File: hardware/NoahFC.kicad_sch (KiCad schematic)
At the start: 44 parts, among them J1 ALE, J11 SCK, J12 MISO, J17 VTX, J18 RESET, J2 ELE, J3 CAM, J4 FTDI, J5 VCC, J6 THR, J7 PPM, J8 GPS, U1 ATmega328, U2 MPU-6050, U4 AMS1117-3.3, U5 MAX7456EUI+, U6 HMC5883L, Y1 16Mhz, Y2 27Mhz

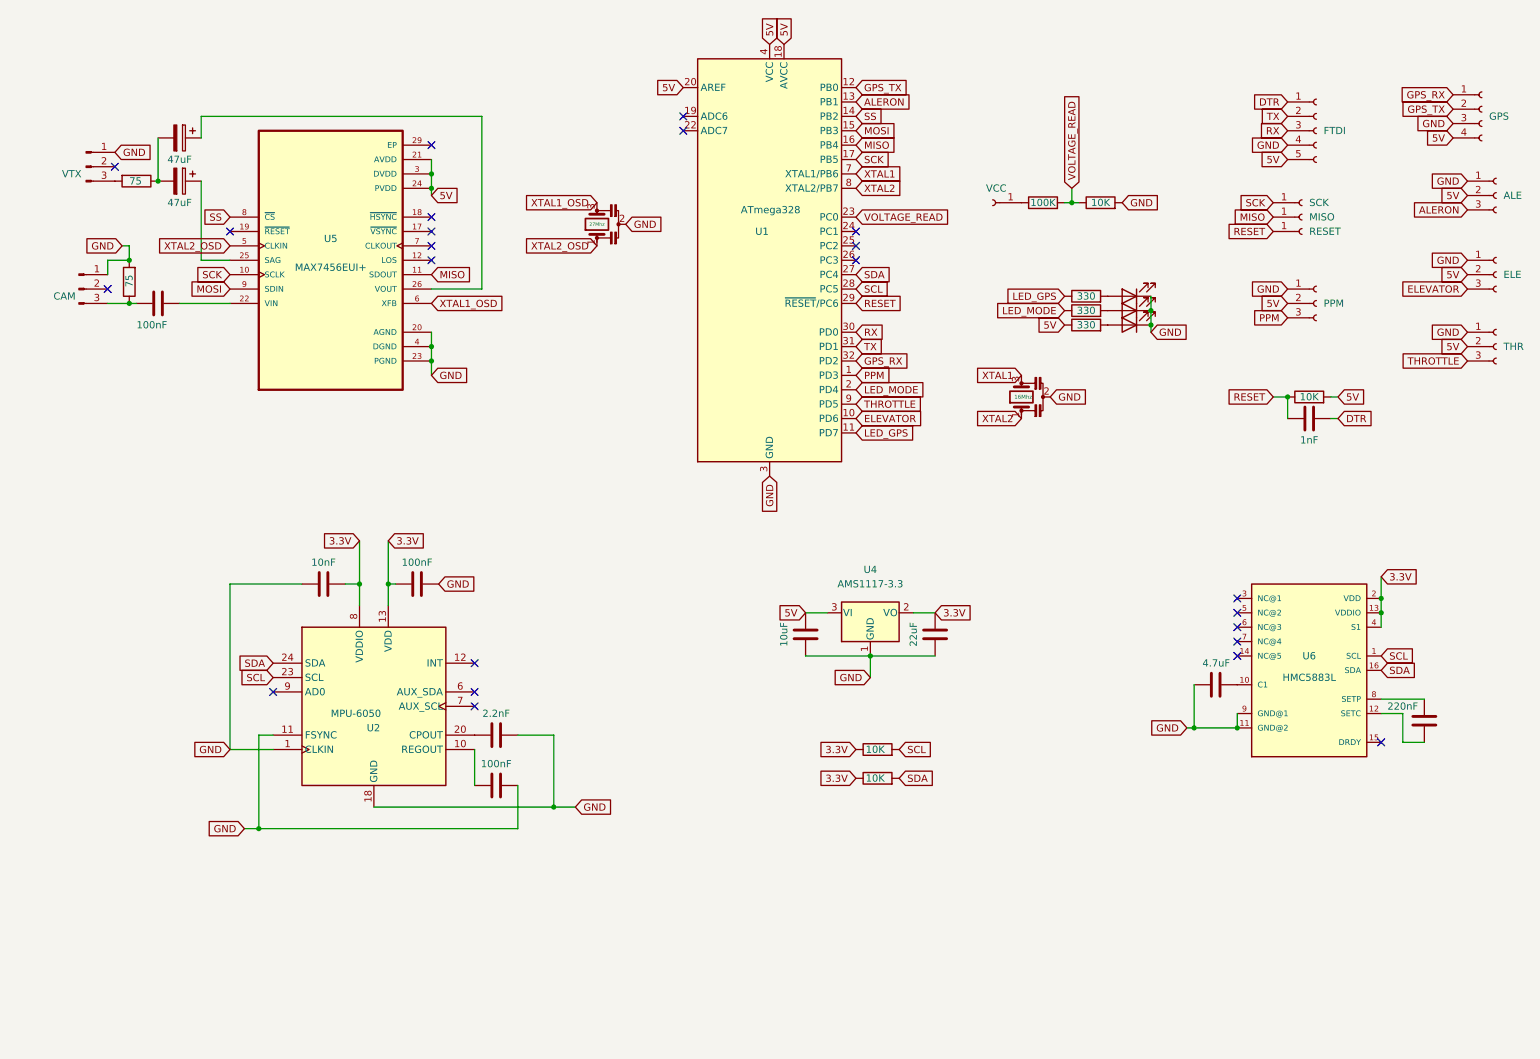
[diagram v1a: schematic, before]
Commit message: rev4 project
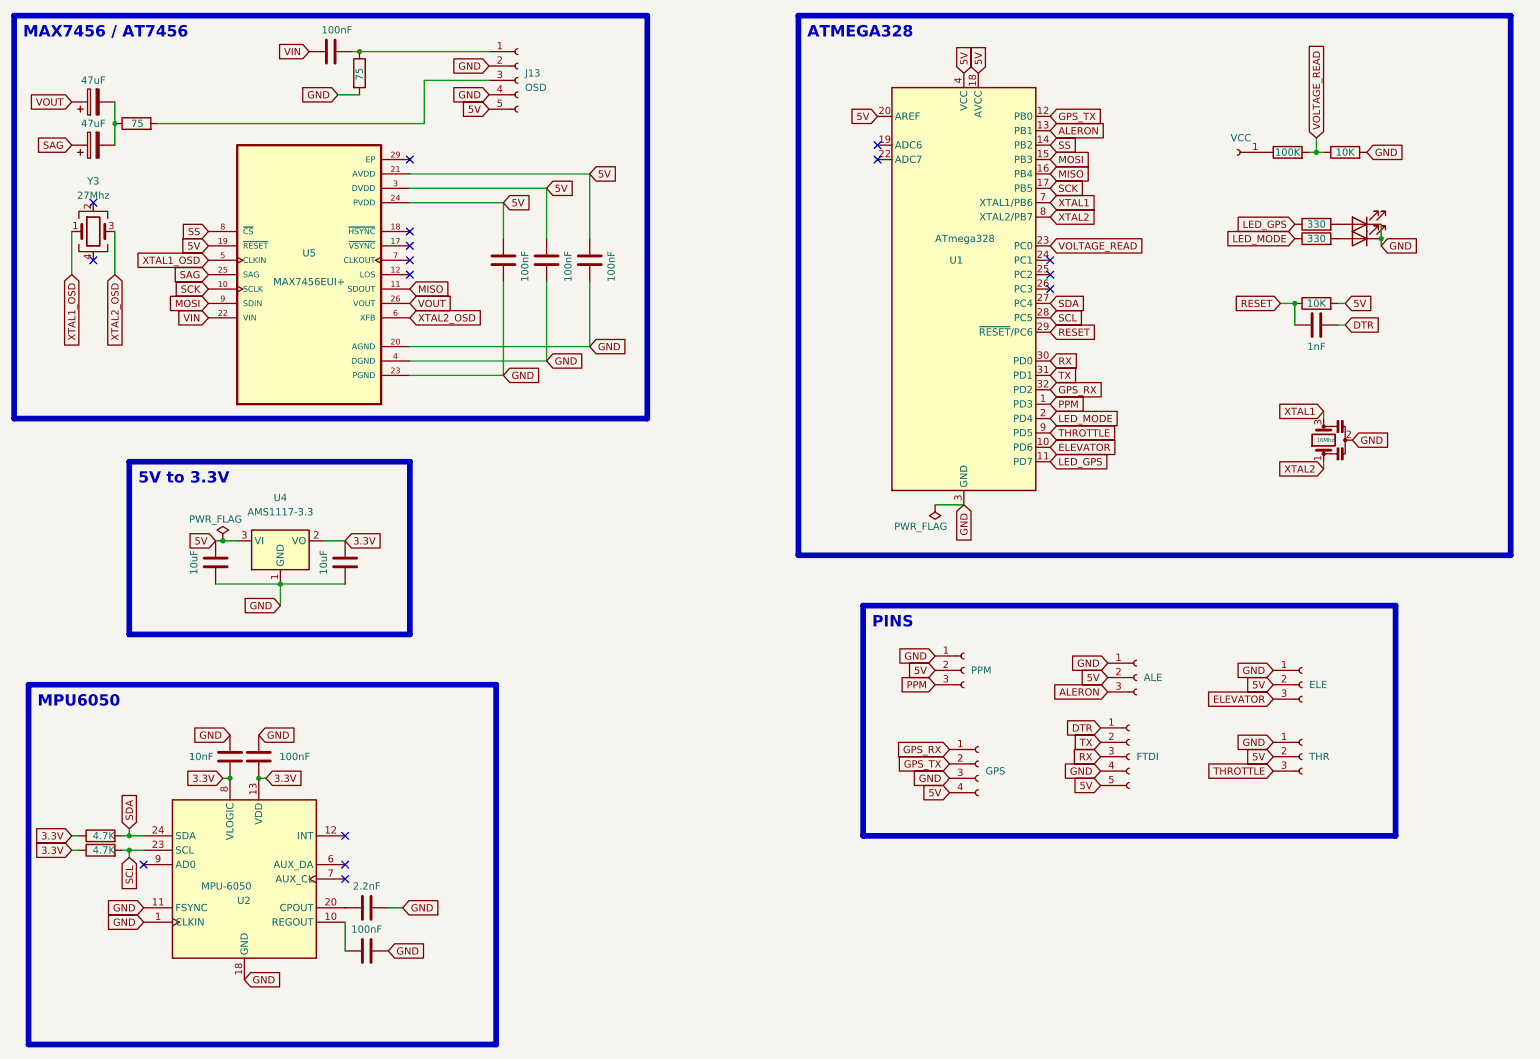
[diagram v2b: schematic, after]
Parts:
- removed C20: 4.7uF, Capacitor_SMD:C_0805_2012Metric, symbol Device:C
- removed C21: 220nF, Capacitor_SMD:C_0805_2012Metric, symbol Device:C
- removed D3: PWR, LED_SMD:LED_0805_2012Metric, symbol Device:LED
- removed J11: SCK, TestPoint:TestPoint_Pad_1.0x1.0mm, symbol Connector:Conn_01x01_Female
- removed J12: MISO, TestPoint:TestPoint_Pad_1.0x1.0mm, symbol Connector:Conn_01x01_Female
- removed J17: VTX, Connector_PinHeader_2.54mm:PinHeader_1x03_P2.54mm_Vertical, symbol Connector:Conn_01x03_Male
- removed J18: RESET, TestPoint:TestPoint_Pad_1.0x1.0mm, symbol Connector:Conn_01x01_Female
- removed J3: CAM, Connector_PinHeader_2.54mm:PinHeader_1x03_P2.54mm_Vertical, symbol Connector:Conn_01x03_Male
- removed R4: 330, Resistor_SMD:R_0805_2012Metric, symbol Device:R
- removed U6: HMC5883L, LPCC-16, symbol HMC5883L:HMC5883L
- removed Y2: 27Mhz, Crystal:Crystal_SMD_3225-4Pin_3.2x2.5mm, symbol Device:Resonator
- added C1, C2, C4: 100nF, Capacitor_SMD:C_0805_2012Metric, symbol Device:C
- added J13: OSD, Connector_JST:JST_SH_BM05B-SRSS-TB_1x05-1MP_P1.00mm_Vertical, symbol Connector:Conn_01x05_Socket
- added Y3: 27Mhz, Crystal:Crystal_SMD_3225-4Pin_3.2x2.5mm, symbol Device:Crystal_GND24
- C11: value 22uF -> 10uF
- J1, J2, J6, J7: symbol Connector:Conn_01x03_Female -> Connector:Conn_01x03_Socket
- J4: footprint Connector_PinHeader_2.54mm:PinHeader_1x05_P2.54mm_Vertical -> Connector_JST:JST_SH_BM05B-SRSS-TB_1x05-1MP_P1.00mm_Vertical; symbol Connector:Conn_01x05_Female -> Connector:Conn_01x05_Socket
- J5: symbol Connector:Conn_01x01_Female -> Connector:Conn_01x01_Socket
- J8: footprint Connector_PinHeader_2.54mm:PinHeader_1x04_P2.54mm_Vertical -> Connector_JST:JST_SH_BM04B-SRSS-TB_1x04-1MP_P1.00mm_Vertical; symbol Connector:Conn_01x04_Female -> Connector:Conn_01x04_Socket
- R7, R8: value 10K -> 4.7K
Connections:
- net 3.3V: now also C6.1, C7.2; no longer C6.2, C7.1
- net 5V: now also U5.19 (~{RESET}), C1.1, C2.1, C4.1, J13.5 (Pin_5)
- net GND: now also C6.2, C7.1, C1.2, C2.2, C4.2, J13.2 (Pin_2), J13.4 (Pin_4); no longer C6.1, C7.2
- net SCL: now also R8.2; no longer R7.2
- net SDA: now also R7.2; no longer R8.2
- net XTAL1_OSD: now also U5.5 (CLKIN), Y3.1; no longer U5.6 (XFB)
- net XTAL2_OSD: now also U5.6 (XFB), Y3.3; no longer U5.5 (CLKIN)
- net at C17.2, R9.1: now also J13.1 (Pin_1)
- net SAG: now reaches C19.1
- net SAG: now also U5.25 (SAG); no longer U5.26 (VOUT)
- net VIN: now reaches C17.1, U5.22 (VIN)
- net at R10.2: now also J13.3 (Pin_3)
- net VOUT: now reaches C18.1
- net VOUT: now also U5.26 (VOUT); no longer U5.25 (SAG)
- no-connect marks 23 -> 16
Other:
- moved on the sheet: U1, U2, U4, U5
